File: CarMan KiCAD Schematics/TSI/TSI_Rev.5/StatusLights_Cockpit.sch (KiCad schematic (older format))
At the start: 18 parts, among them Q3 ZVP1320F, U1 RDE03110S12, U11 TLP293, U13 TLP293

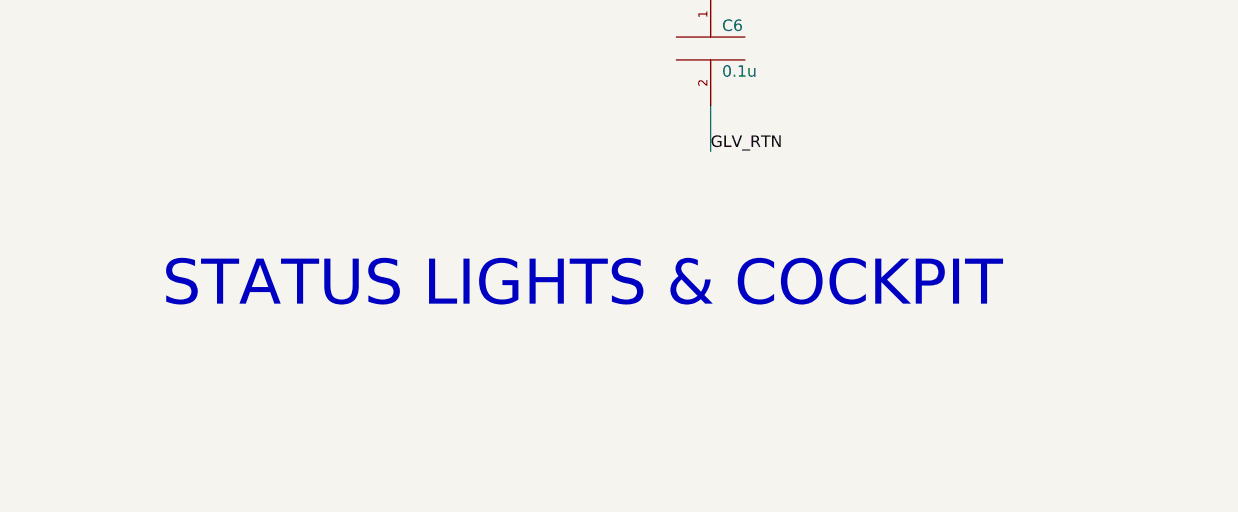
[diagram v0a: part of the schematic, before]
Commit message: - Updating TSI
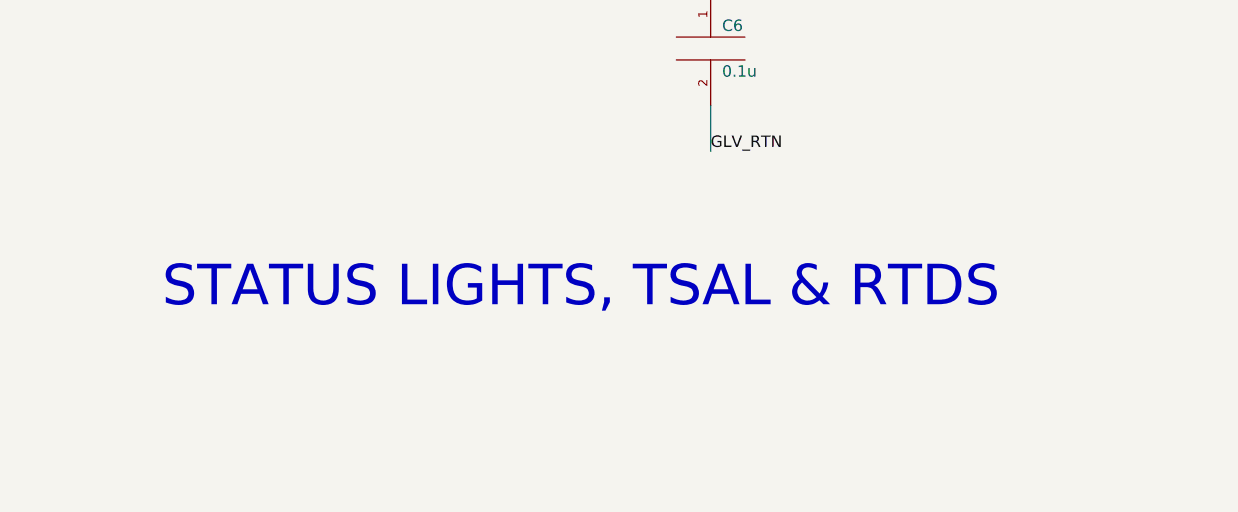
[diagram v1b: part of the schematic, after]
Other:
- note added: "STATUS LIGHTS, TSAL & RTDS"
- note removed: "STATUS LIGHTS & COCKPIT"
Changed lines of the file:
@@
 Wire Wire Line
 	5600 1550 5400 1550
-Text Notes 7100 6950 0    197  ~ 0
-STATUS LIGHTS & COCKPIT
+Text Notes 7100 6950 0    177  ~ 0
+STATUS LIGHTS, TSAL & RTDS
 Text HLabel 1150 1800 0    50   Input ~ 0
 RTDS
